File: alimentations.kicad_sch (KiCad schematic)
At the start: 15 parts, among them IC1 5v to 3.3v, J1 connecteur batterie, U2 MAX20077ATCA/VY+, U3 3.3v to 1.8v

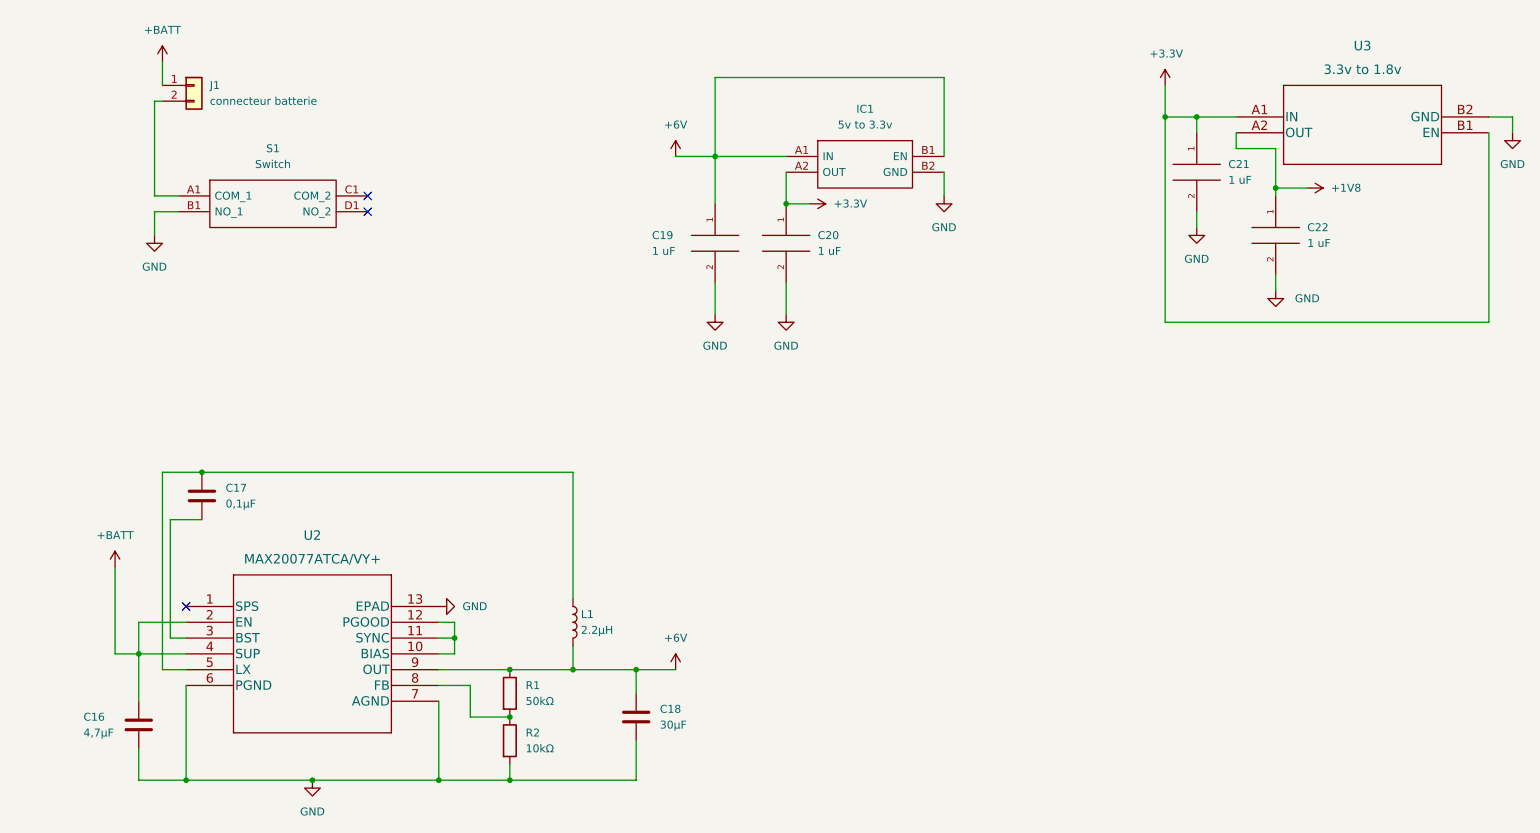
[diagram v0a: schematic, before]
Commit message: merge files for presentation
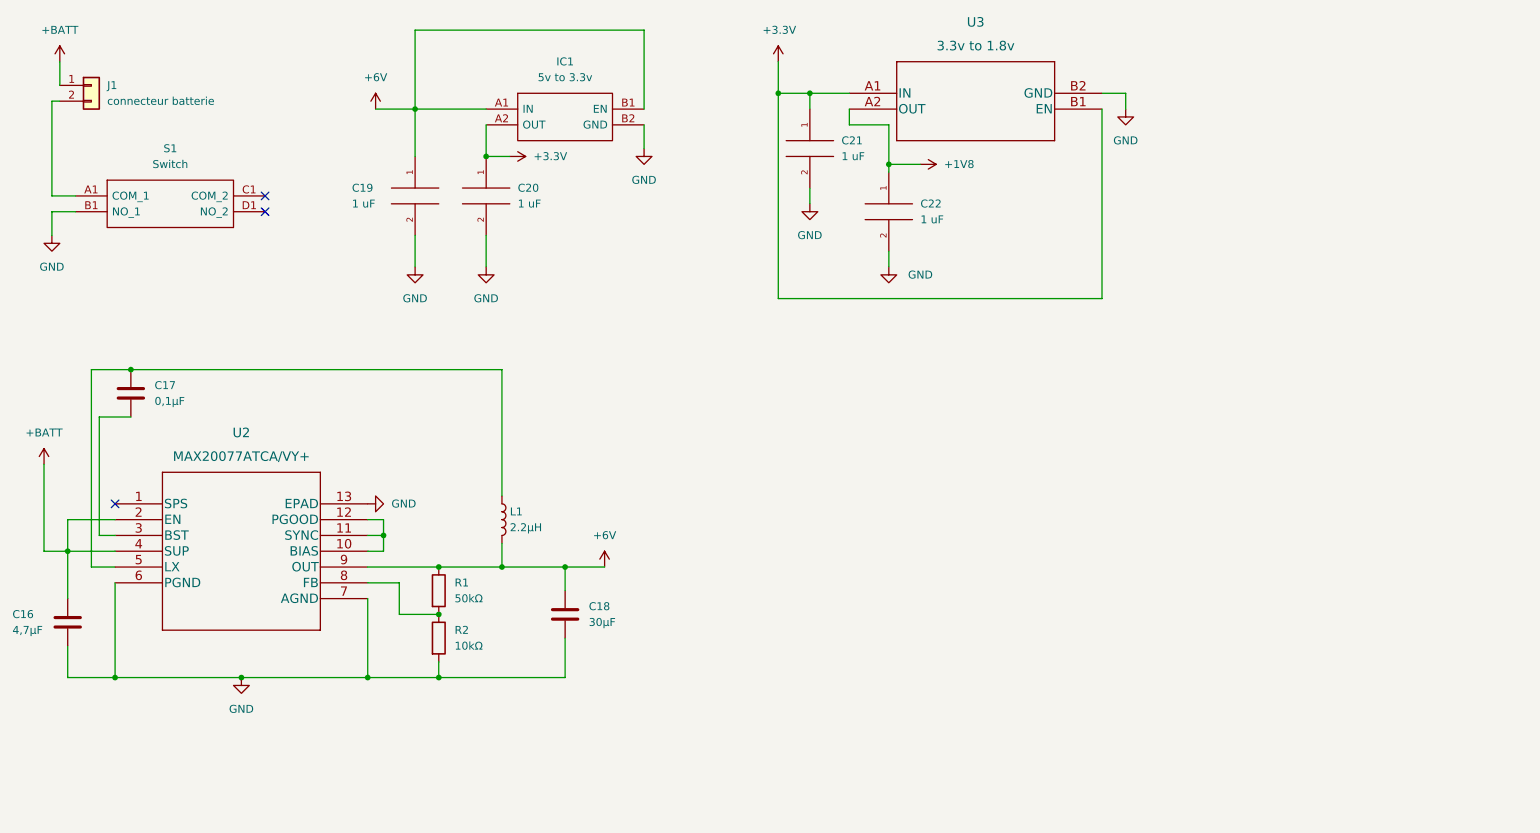
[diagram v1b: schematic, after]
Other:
- moved on the sheet: C16, C17, C18, C19, C20, C21, C22, IC1, J1, L1, R1, R2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
